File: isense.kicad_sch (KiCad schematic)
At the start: 29 parts, among them U2 OPA551U, U3 OPA551U, U4 TLV9301

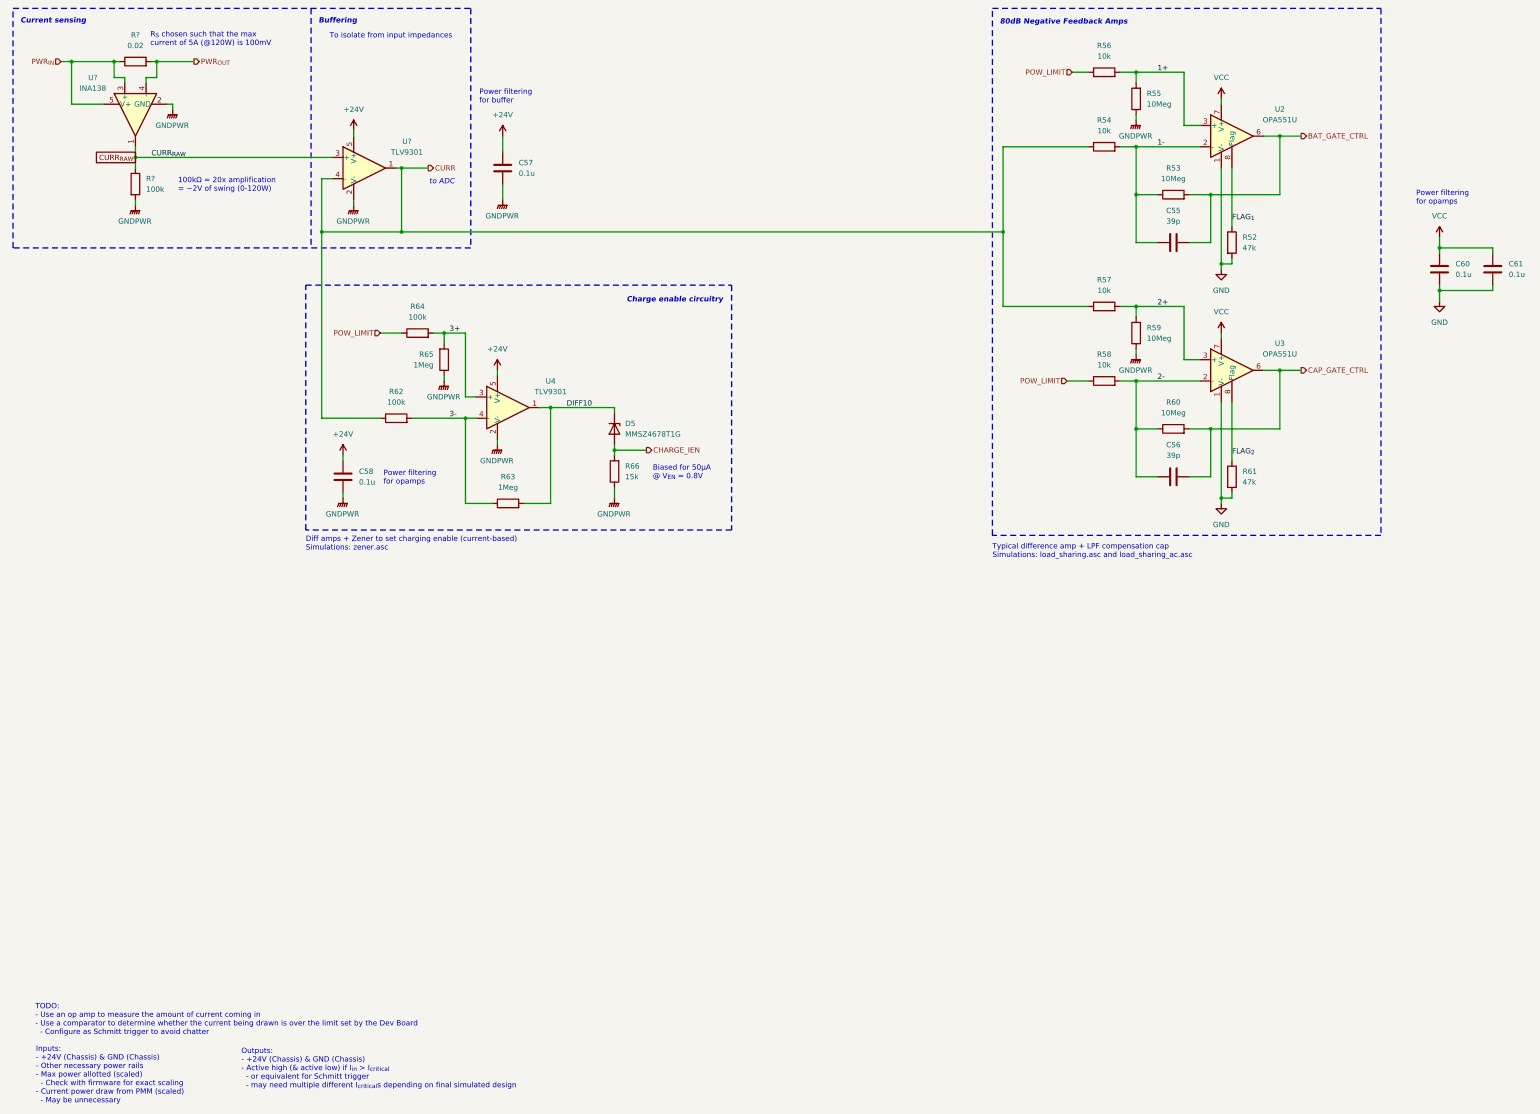
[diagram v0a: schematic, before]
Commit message: Redesign housekeeping supplies
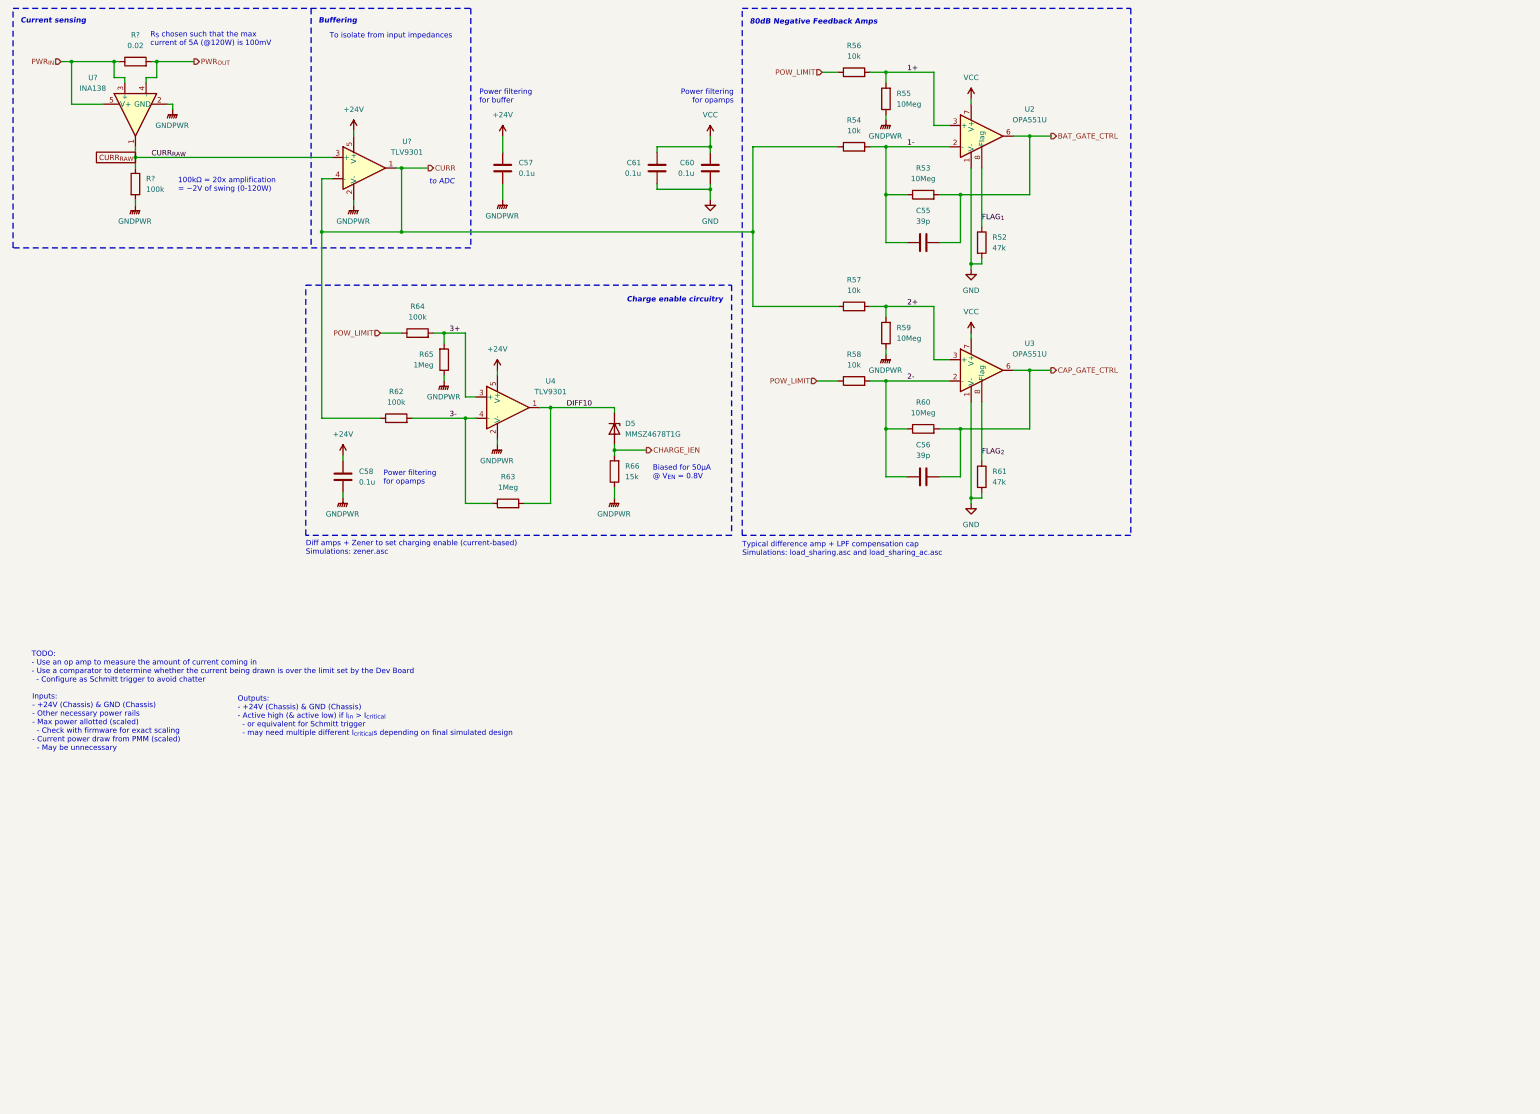
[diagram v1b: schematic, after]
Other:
- moved on the sheet: C55, C56, C60, C61, R52, R53, R54, R55, R56, R57, R58, R59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
